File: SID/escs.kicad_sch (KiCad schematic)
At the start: 0 parts

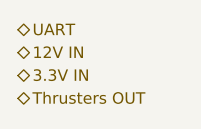
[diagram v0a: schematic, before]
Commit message: Feat(SID): basically complete
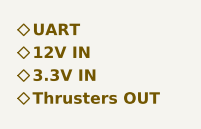
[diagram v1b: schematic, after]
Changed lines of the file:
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@@
-(kicad_sch (version 20230819) (generator eeschema)
-  (paper "A4")
-  (hierarchical_label "12V IN" (shape bidirectional) (at 109.22 93.98 0) (fields_autoplaced)
-    (effects (font (size 1.27 1.27)) (justify left))
-  )
-  (hierarchical_label "3.3V IN" (shape bidirectional) (at 109.22 96.52 0) (fields_autoplaced)
-    (effects (font (size 1.27 1.27)) (justify left))
-  )
-  (hierarchical_label "UART" (shape bidirectional) (at 109.22 91.44 0) (fields_autoplaced)
-    (effects (font (size 1.27 1.27)) (justify left))
-  )
-  (hierarchical_label "Thrusters OUT" (shape bidirectional) (at 109.22 99.06 0) (fields_autoplaced)
-    (effects (font (size 1.27 1.27)) (justify left))
-  )
+(kicad_sch
+	(version 20240101)
+	(generator "eeschema")
+	(generator_version "8.99")
+	(paper "A4")
+	(hierarchical_label "12V IN"
+		(shape bidirectional)
+		(at 109.22 93.98 0)
+		(fields_autoplaced yes)
+		(effects
+			(font
+				(face "JetBrains Mono")
+				(size 1.27 1.27)
+				(thickness 0.254)
+				(bold yes)
+			)
+			(justify left)
+		)
+	)
+	(hierarchical_label "3.3V IN"
+		(shape bidirectional)
+		(at 109.22 96.52 0)
+		(fields_autoplaced yes)
+		(effects
+			(font
+				(face "JetBrains Mono")
+				(size 1.27 1.27)
+				(thickness 0.254)
+				(bold yes)
+			)
+			(justify left)
+		)
+	)
+	(hierarchical_label "UART"
+		(shape bidirectional)
+		(at 109.22 91.44 0)
+		(fields_autoplaced yes)
+		(effects
+			(font
+				(face "JetBrains Mono")
+				(size 1.27 1.27)
+				(thickness 0.254)
+				(bold yes)
+			)
+			(justify left)
+		)
+	)
+	(hierarchical_label "Thrusters OUT"
+		(shape bidirectional)
+		(at 109.22 99.06 0)
+		(fields_autoplaced yes)
+		(effects
+			(font
+				(face "JetBrains Mono")
+				(size 1.27 1.27)
+				(thickness 0.254)
+				(bold yes)
+			)
+			(justify left)
+		)
+	)
 )
